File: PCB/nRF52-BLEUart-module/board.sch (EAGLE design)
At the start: 44 parts, among them J1 USB-A_PTH_MALE, U1 CH340E, U2 NRF52832, Y1 32MHz_2016, Y2 32.768kHz

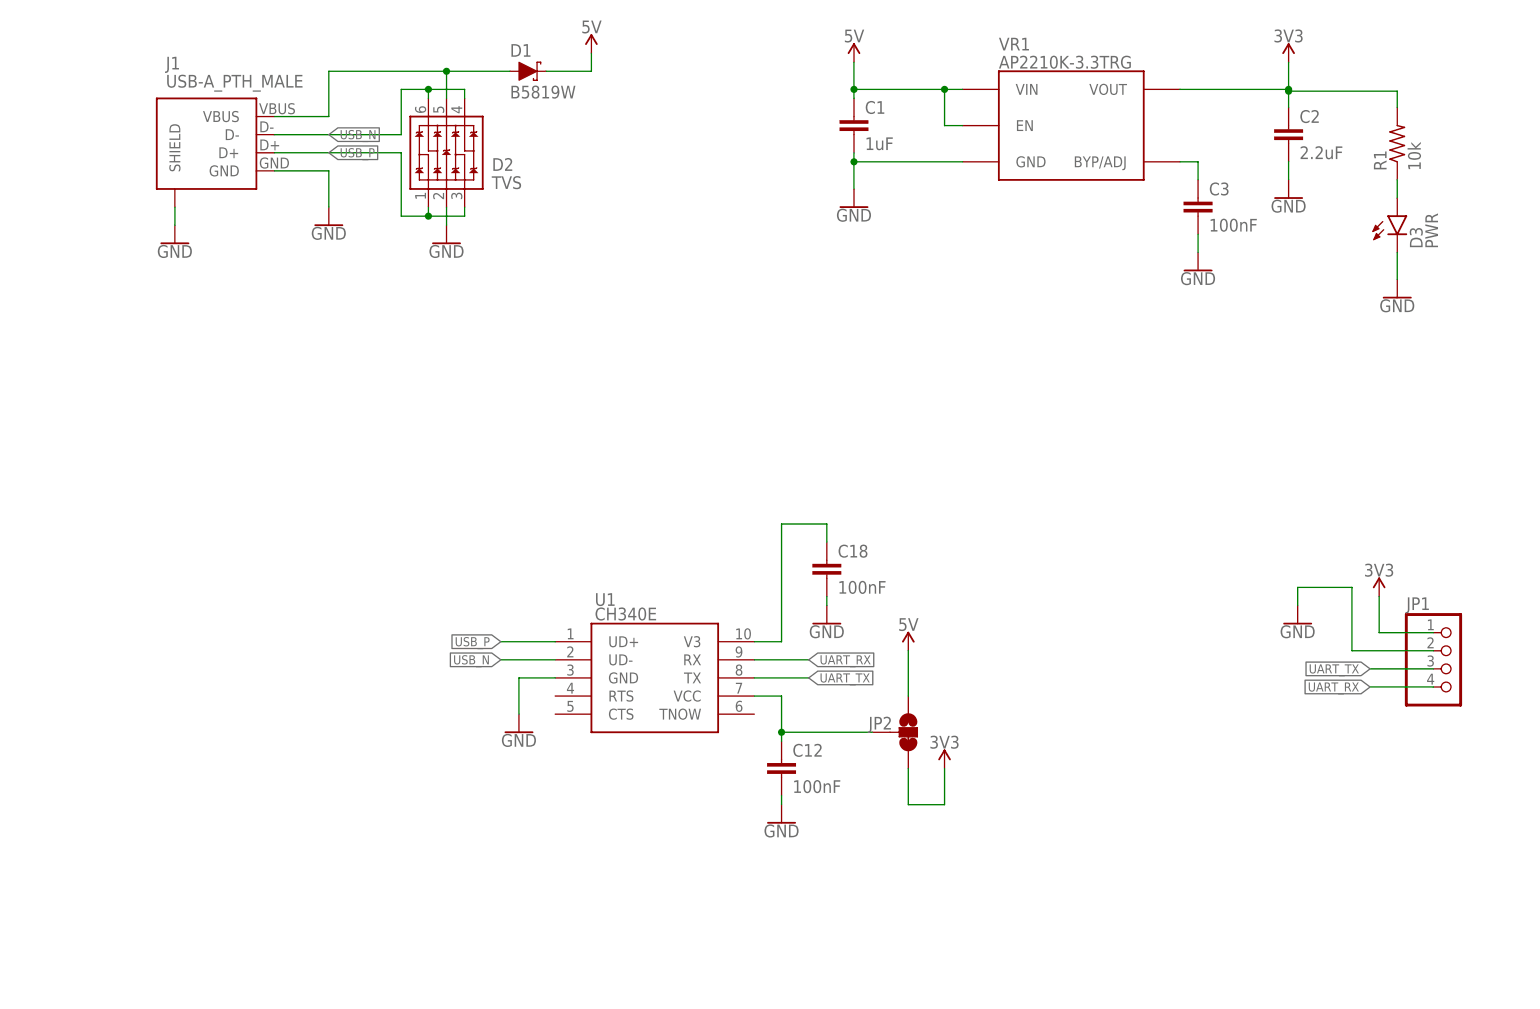
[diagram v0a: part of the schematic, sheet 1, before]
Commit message: artwork partially done, layout update
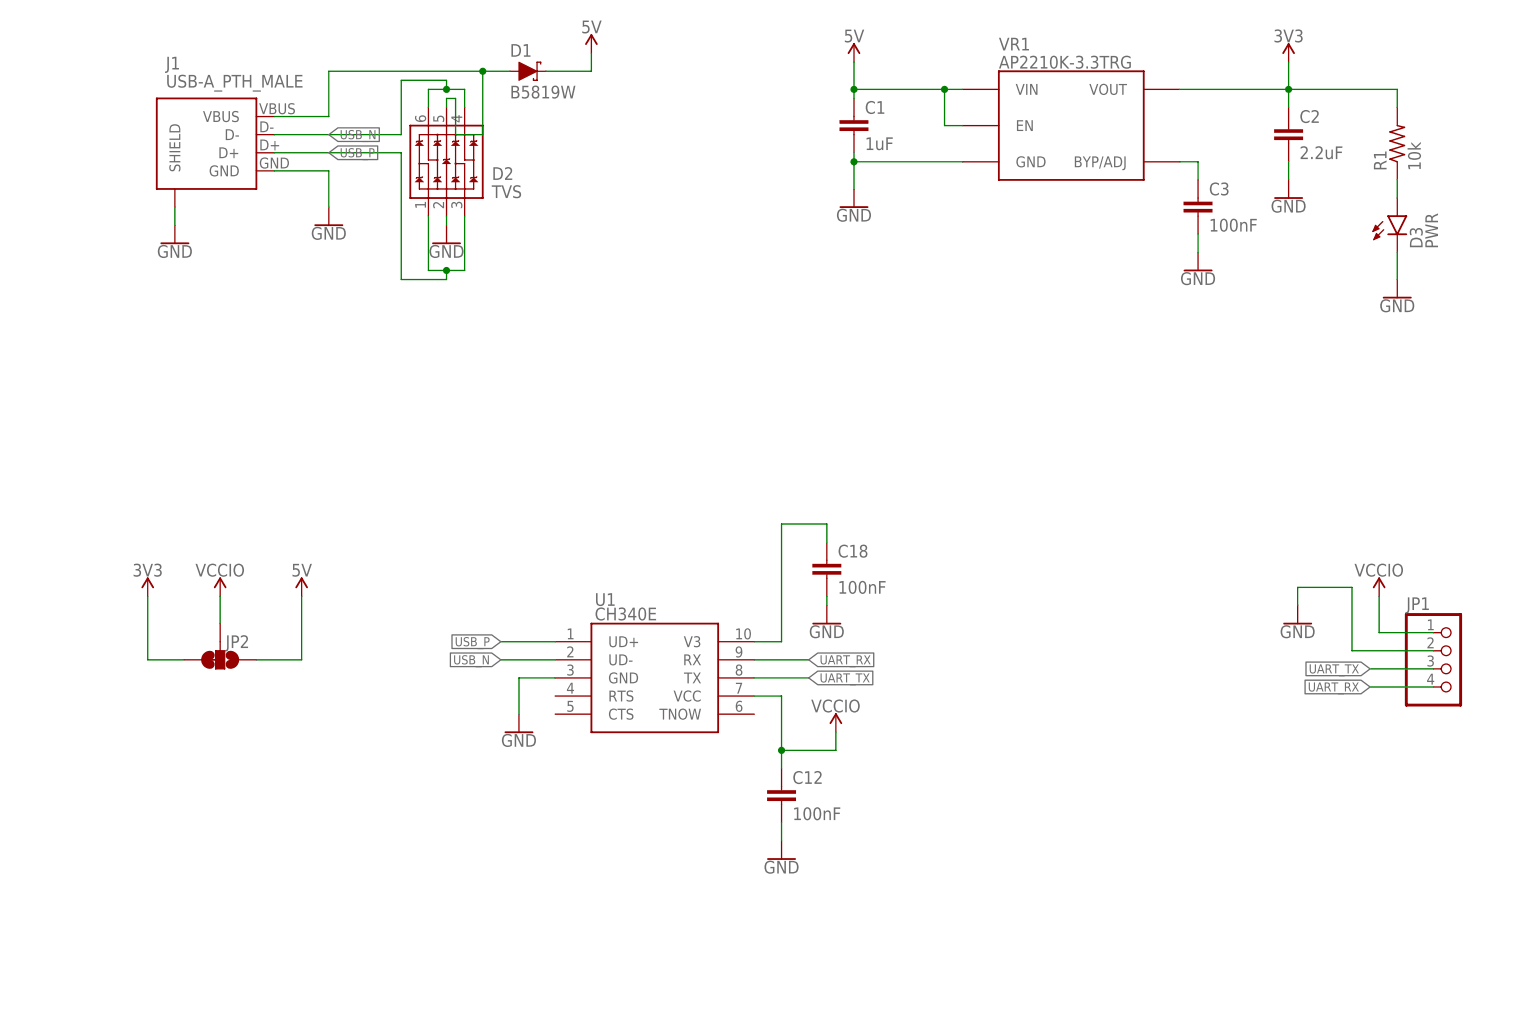
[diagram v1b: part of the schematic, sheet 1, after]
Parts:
- added C19: TP, angrypig7-RCL:C-NON-POLC0603
- JP1: value V G Rx Tx -> V G Tx Rx
- JP3, JP4: device angrypig7-Connectors-PinHeads:PINHD-1X6 -> angrypig7-Connectors-PinHeads:PINHD-1X5-NOSILK
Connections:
- net N$2 renamed USB_IN
- removed net N$15: C12.1, JP2.2, U1.VCC
- new net VCCIO: C12.1, JP1.1, JP2.2, U1.VCC
- net 3V3: no longer JP1.1
- net GND: now also C19.2
- net RF-1: now also C19.1
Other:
- moved on the sheet: C12, C15, C16, D2, JP2, L1
